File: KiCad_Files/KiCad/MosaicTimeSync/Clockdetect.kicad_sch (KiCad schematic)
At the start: 12 parts, among them Q1 NTK3139PT5G, U2 TLV3511DCKR, U5 SN74LVC1G3157DRLR

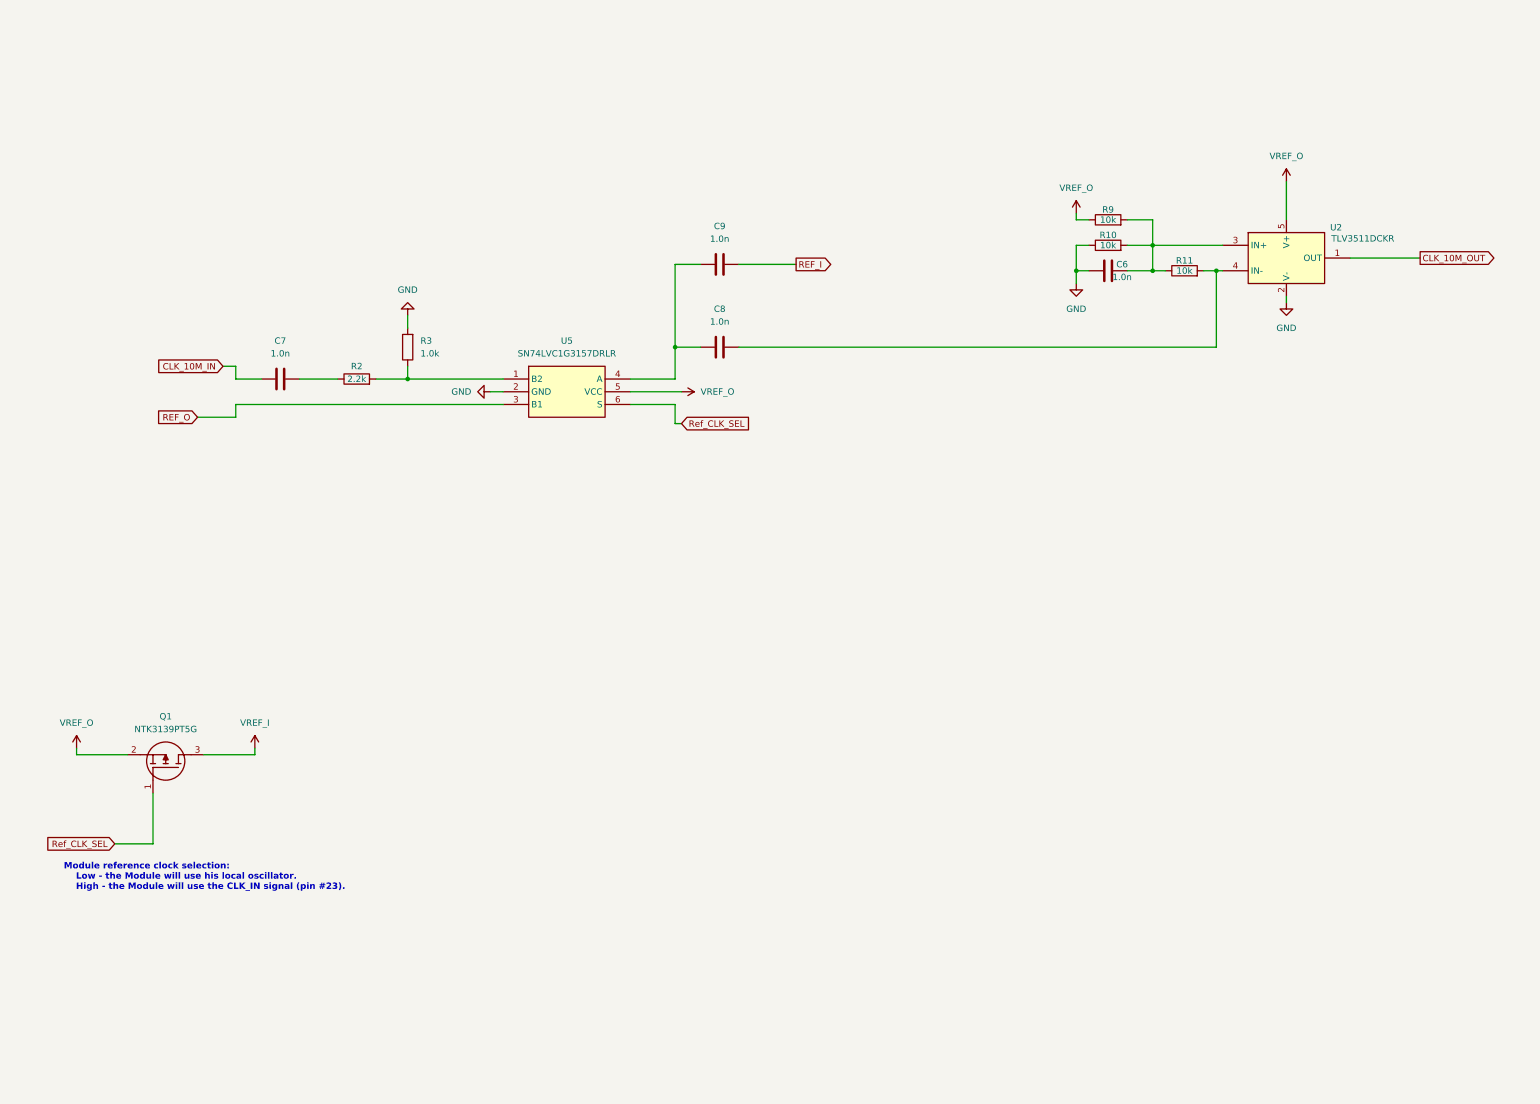
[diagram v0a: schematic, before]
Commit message: KiCad update
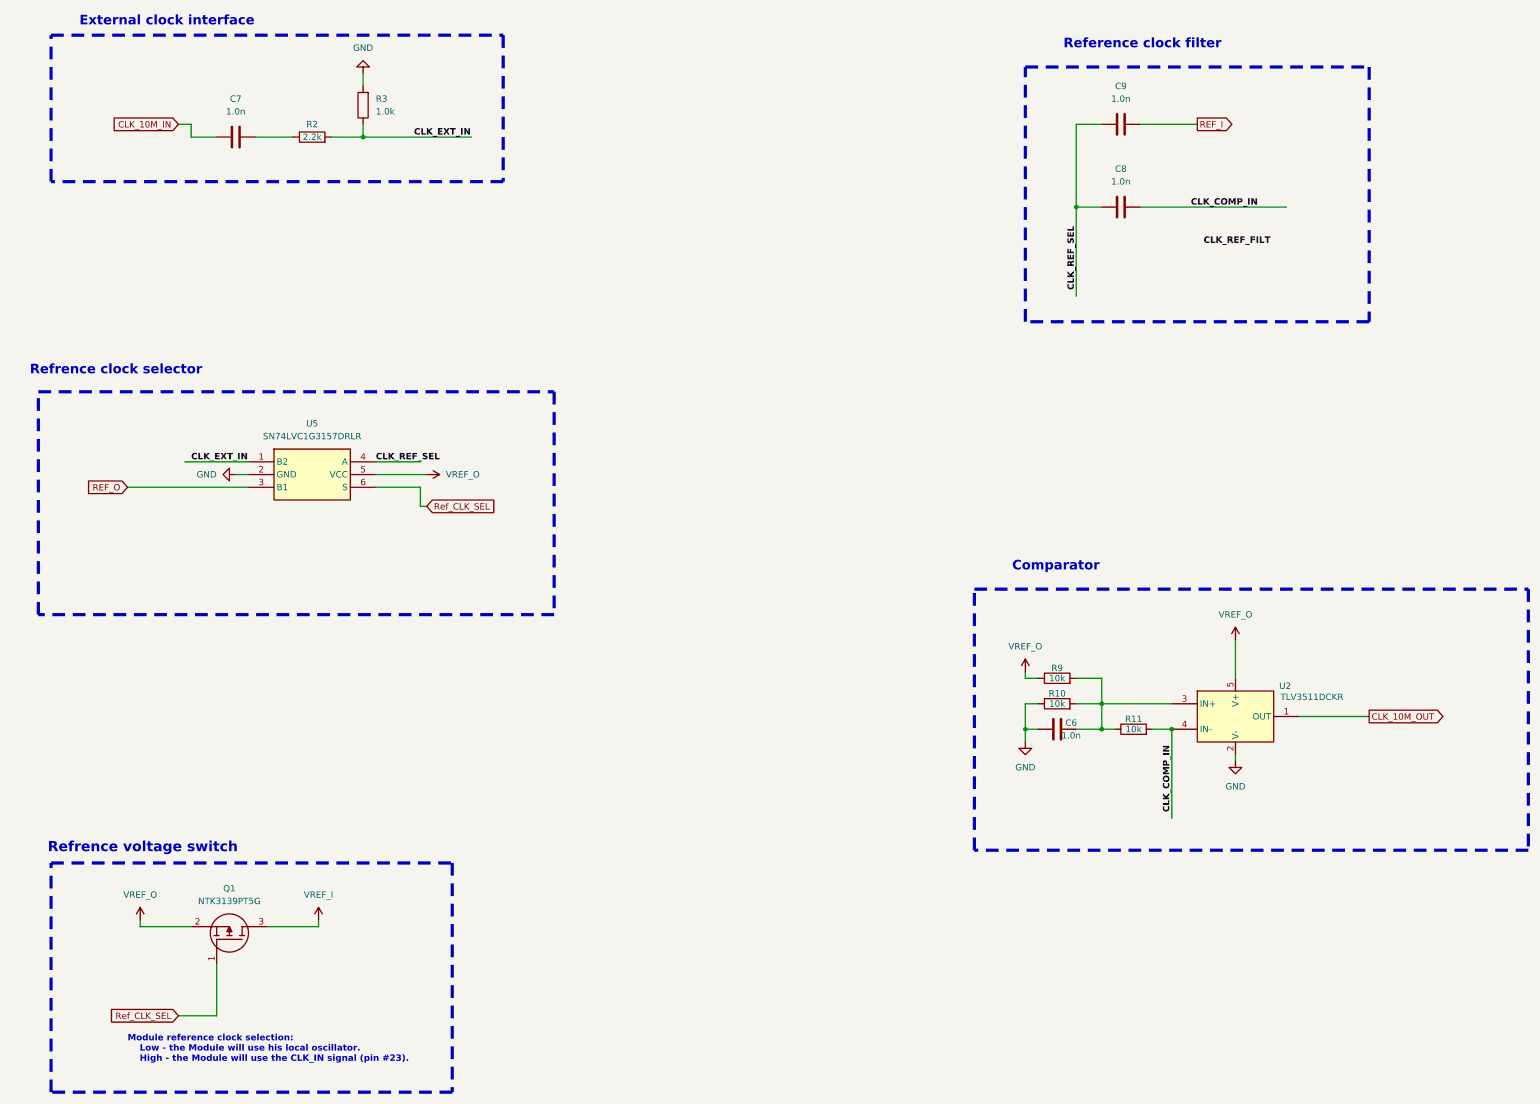
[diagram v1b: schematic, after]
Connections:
- net CLK_COMP_IN: now reaches C8.2, R11.2, U2.4 (IN-)
- net CLK_REF_SEL: now reaches C8.1, C9.1, U5.4 (A)
- net CLK_EXT_IN: now reaches R2.2, R3.1, U5.1 (B2)
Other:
- note added: "Comparator"
- note added: "External clock interface"
- note added: "Reference clock filter"
- note added: "Refrence clock selector"
- note added: "Refrence voltage switch"
- title: M2_mosaic G5-T_Module  -> MosaicTimeSync
- moved on the sheet: C6, C7, C8, C9, Q1, R10, R11, R2, R3, R9, U2, U5
